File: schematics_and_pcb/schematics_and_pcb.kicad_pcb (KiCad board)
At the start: 2 copper layers, 47 x 89.8 mm, 59 parts, among them J1 RND 205-00623, J2 RND 205-00627, J3 Motor con, J5 Conn_01x04_Male, J6 USB_OTG_custom, Q1 PMV213SN, SW1 RND 210-00210, U1 LP2985IM5-2.0/NOPB, U2 TS3480CX33 RFG, U3 PWM3389DM-T3QU, U4 STM32F401RBTx, Y1 YLFXTAL029370

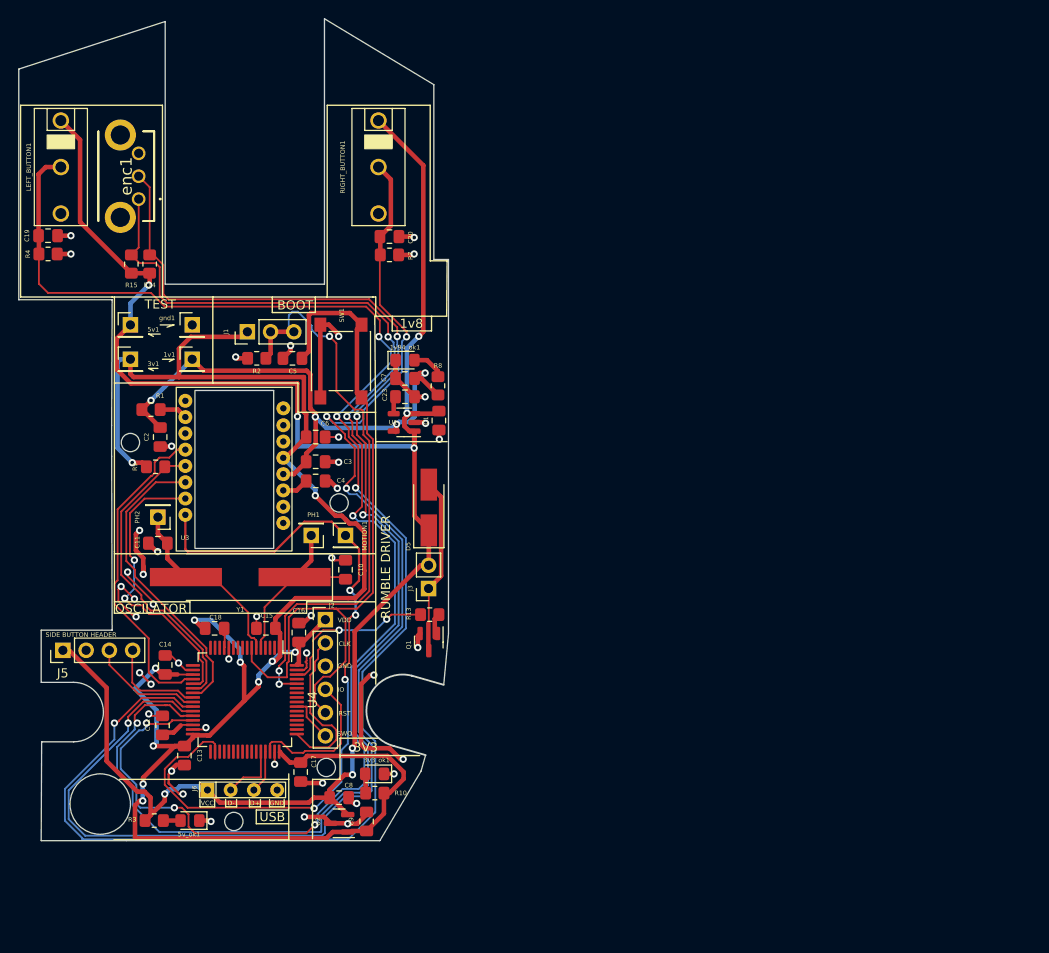
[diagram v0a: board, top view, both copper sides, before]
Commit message: probs final version
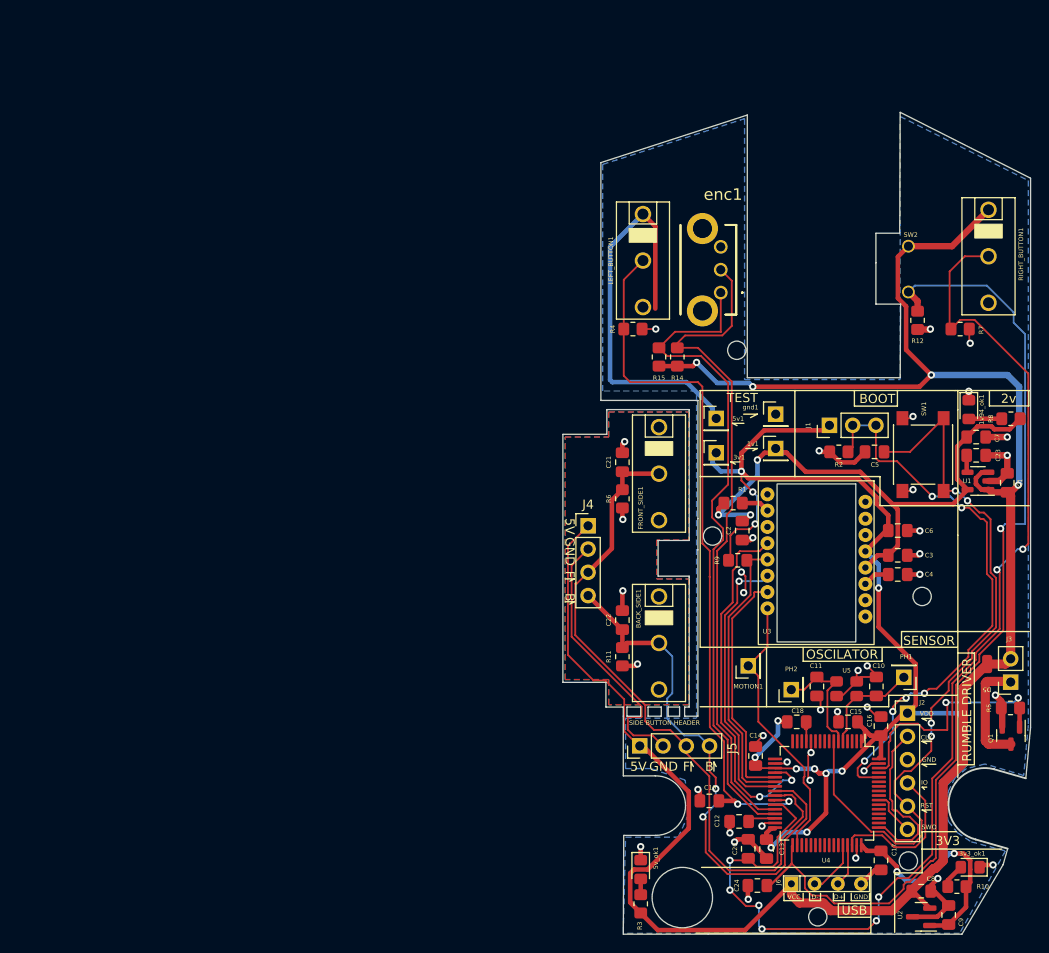
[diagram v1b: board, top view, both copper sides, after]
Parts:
- removed G***: LOGO, LOGO
- removed R13: 1K, Resistor_SMD:R_0805_2012Metric_Pad1.20x1.40mm_HandSolder
- removed Y1: YLFXTAL029370, Crystal:Crystal_SMD_HC49-SD_HandSoldering
- added BACK_SIDE1: D2F-01F, mouse:D2F-01F, F.Cu at (89.8, 82.5)
- added C21: 10u, Capacitor_SMD:C_0805_2012Metric_Pad1.18x1.45mm_HandSolder, F.Cu at (85.8, 62.8)
- added C22: 10u, Capacitor_SMD:C_0805_2012Metric_Pad1.18x1.45mm_HandSolder, F.Cu at (85.8, 80.0)
- added C24: 10u, Capacitor_SMD:C_0805_2012Metric_Pad1.18x1.45mm_HandSolder, F.Cu at (100.5, 109.0)
- added FRONT_SIDE1: D2F-01F, mouse:D2F-01F, F.Cu at (89.8, 64.0)
- added J4: Conn_01x04_Male, Connector_PinHeader_2.54mm:PinHeader_1x04_P2.54mm_Vertical, F.Cu at (82.0, 69.7)
- added R11: 4.7k, Resistor_SMD:R_0805_2012Metric_Pad1.20x1.40mm_HandSolder, F.Cu at (85.8, 84.0)
- added R12: 4.7k, Resistor_SMD:R_0805_2012Metric_Pad1.20x1.40mm_HandSolder, F.Cu at (118.0, 47.2)
- added R5: 10k, Resistor_SMD:R_0805_2012Metric_Pad1.20x1.40mm_HandSolder, F.Cu at (128.2, 89.6)
- added R6: 4.7k, Resistor_SMD:R_0805_2012Metric_Pad1.20x1.40mm_HandSolder, F.Cu at (85.8, 66.8)
- added SW2: SW_Push, mouse:evqP0E07, F.Cu at (117.0, 41.6)
- added U5: LFXTAL055951, mouse:LFXTAL055951, F.Cu at (110.2, 87.5)
- C10, C11: value 22p -> 18p
- C4: value 4u -> 4u7
- D5: value S1A -> SS16HE; footprint Diode_SMD:D_SMA_Handsoldering -> mouse:SOD-323HE
- J1: value RND 205-00623 -> RND 205-00624
- Q1: value PMV213SN -> TSM2308CX RFG
- moved C19 95.0 mm to (95.2, 99.8), turned to 0 degrees
- moved C20 77.5 mm to (99.5, 105.0), turned to -90 degrees
- moved C11 73.7 mm to (107.0, 87.2), turned to 90 degrees
- moved PH2 71.7 mm to (104.2, 87.6), turned to 90 degrees
- moved RIGHT_BUTTON1 67.4 mm to (125.8, 40.2)
- moved PH1 66.6 mm to (116.5, 86.2)
- moved 3v3_ok1 65.9 mm to (123.8, 107.0)
- moved C14 65.3 mm to (100.3, 94.8)
- moved 3v1 64.8 mm to (96.0, 61.7)
- moved 5v1 64.8 mm to (96.0, 58.0)
- moved J6 64.6 mm to (106.8, 111.4)
- moved 1v1 64.5 mm to (102.5, 61.2)
- moved gnd1 64.5 mm to (102.5, 57.5)
- moved R4 64.4 mm to (86.9, 48.2)
- moved C13 64.4 mm to (101.5, 105.0)
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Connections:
- Q1 pad 1: Net-(Q1-Pad1) -> RUMBLE
- U4 pad 33: unconnected-(U4-Pad33) -> WHEEL_BUTTON
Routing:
- net WHEEL_BUTTON: track 0.00 -> 107.6 mm, vias 0 -> 1
- net LEFT_STATE: track 175.7 -> 79.8 mm, vias 4 -> 2
- net PHASE_A: track 147.9 -> 72.5 mm, vias 4 -> 0
- net PHASE_B: track 144.7 -> 73.5 mm, vias 6 -> 0
- net FRONT_STATE: track 12.4 -> 74.7 mm
- net +5V: track 212.5 -> 273.2 mm, vias 8 -> 4
- net MOTION: track 84.4 -> 30.2 mm, vias 4 -> 0
- net BACK_STATE: track 10.8 -> 60.7 mm, vias 0 -> 2
- net VDDIO: track 211.9 -> 171.5 mm, vias 11 -> 14
- net RIGHT_STATE: track 143.5 -> 127.7 mm, vias 4 -> 8
- net GND: track 105.8 -> 119.4 mm, vias 44 -> 39
- net PH0: track 20.2 -> 11.6 mm
- net RUMBLE: track 17.9 -> 25.9 mm
- net Net-(D5-Pad2): track 19.4 -> 12.1 mm
- net PH1: track 20.6 -> 13.5 mm
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- added copper zone on F.Cu, net +5V
- added copper zone on B.Cu, net GND
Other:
- board size 47 x 89.8 mm -> 51.1 x 89.8 mm
- board text added: "2v"
- board text added: "5V"
- board text added: "B"
- board text added: "F"
- board text added: "SENSOR"
- board text removed: "1v8"
- board text removed: "Awesome gaming mouse"
- board text removed: "MAIN MOUSE BOARD"
- board text removed: "Mouse Logo Vectors by Vecteezy"
